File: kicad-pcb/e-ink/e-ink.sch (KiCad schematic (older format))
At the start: 0 parts

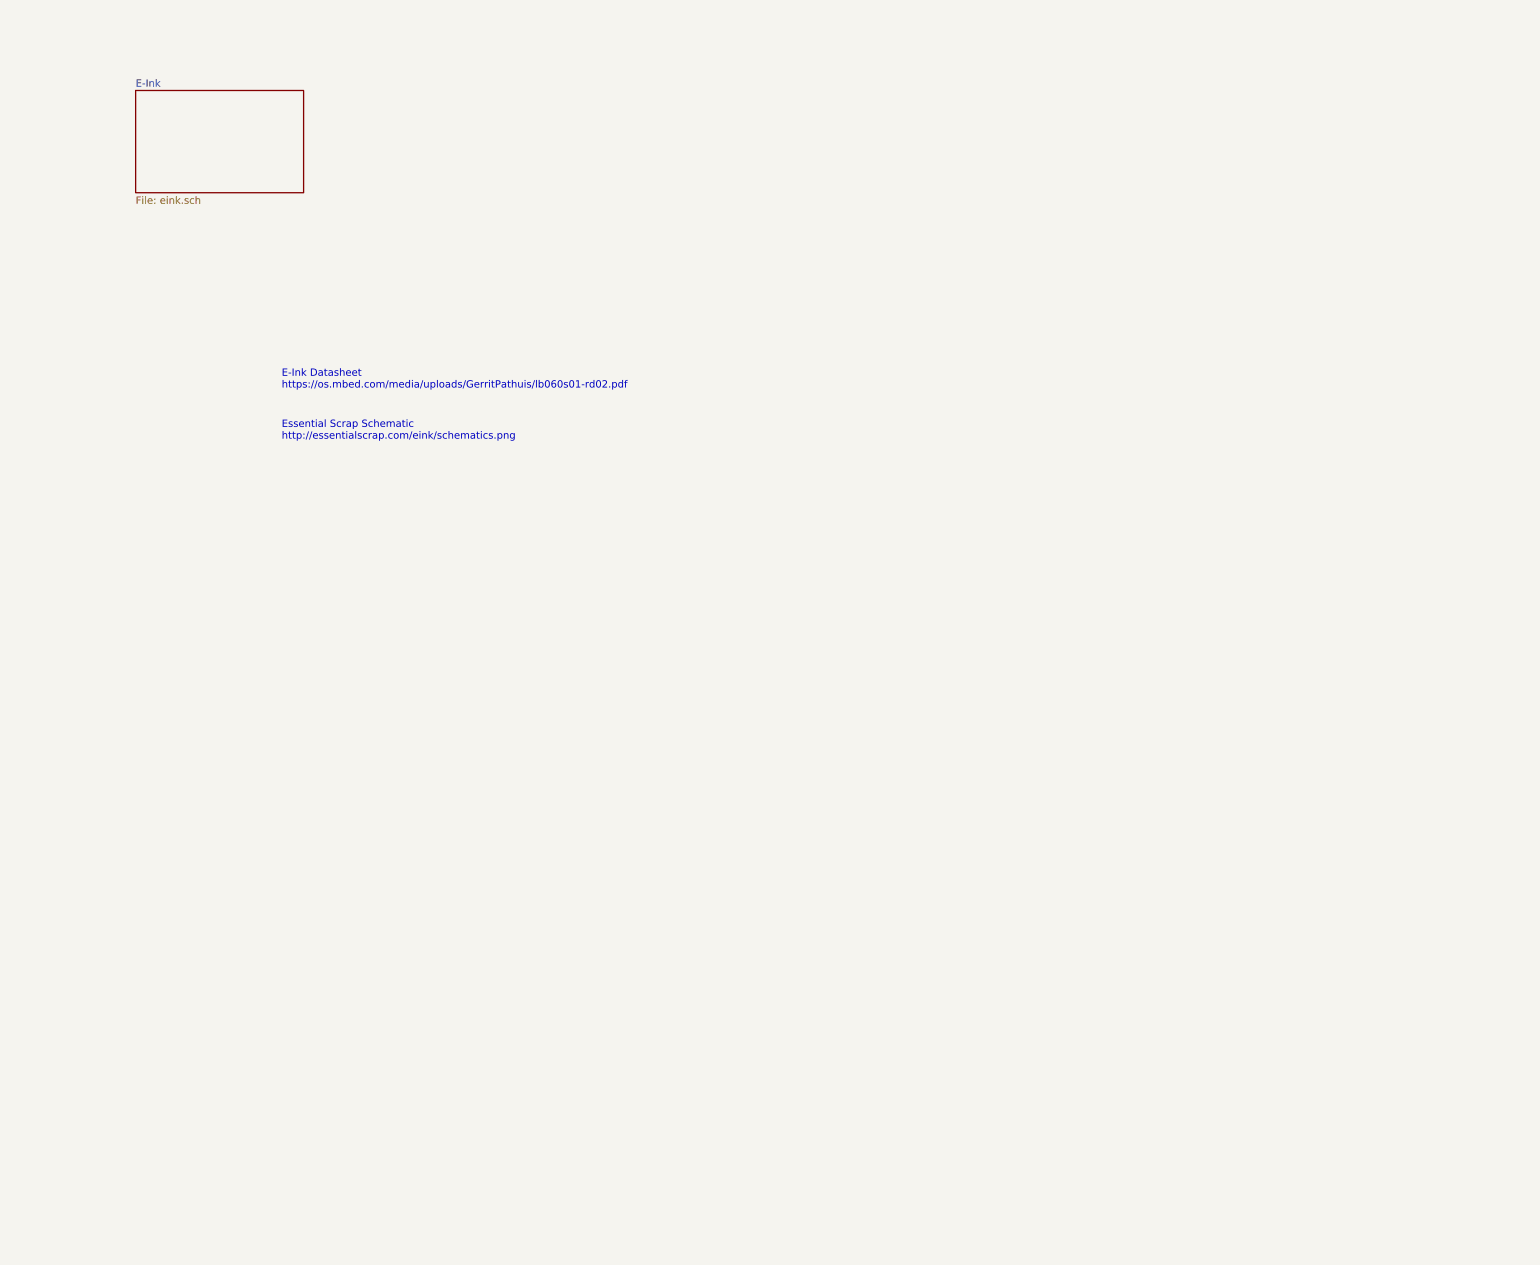
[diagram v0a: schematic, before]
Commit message: recovered from an unplanned poweroff, and removed backup files
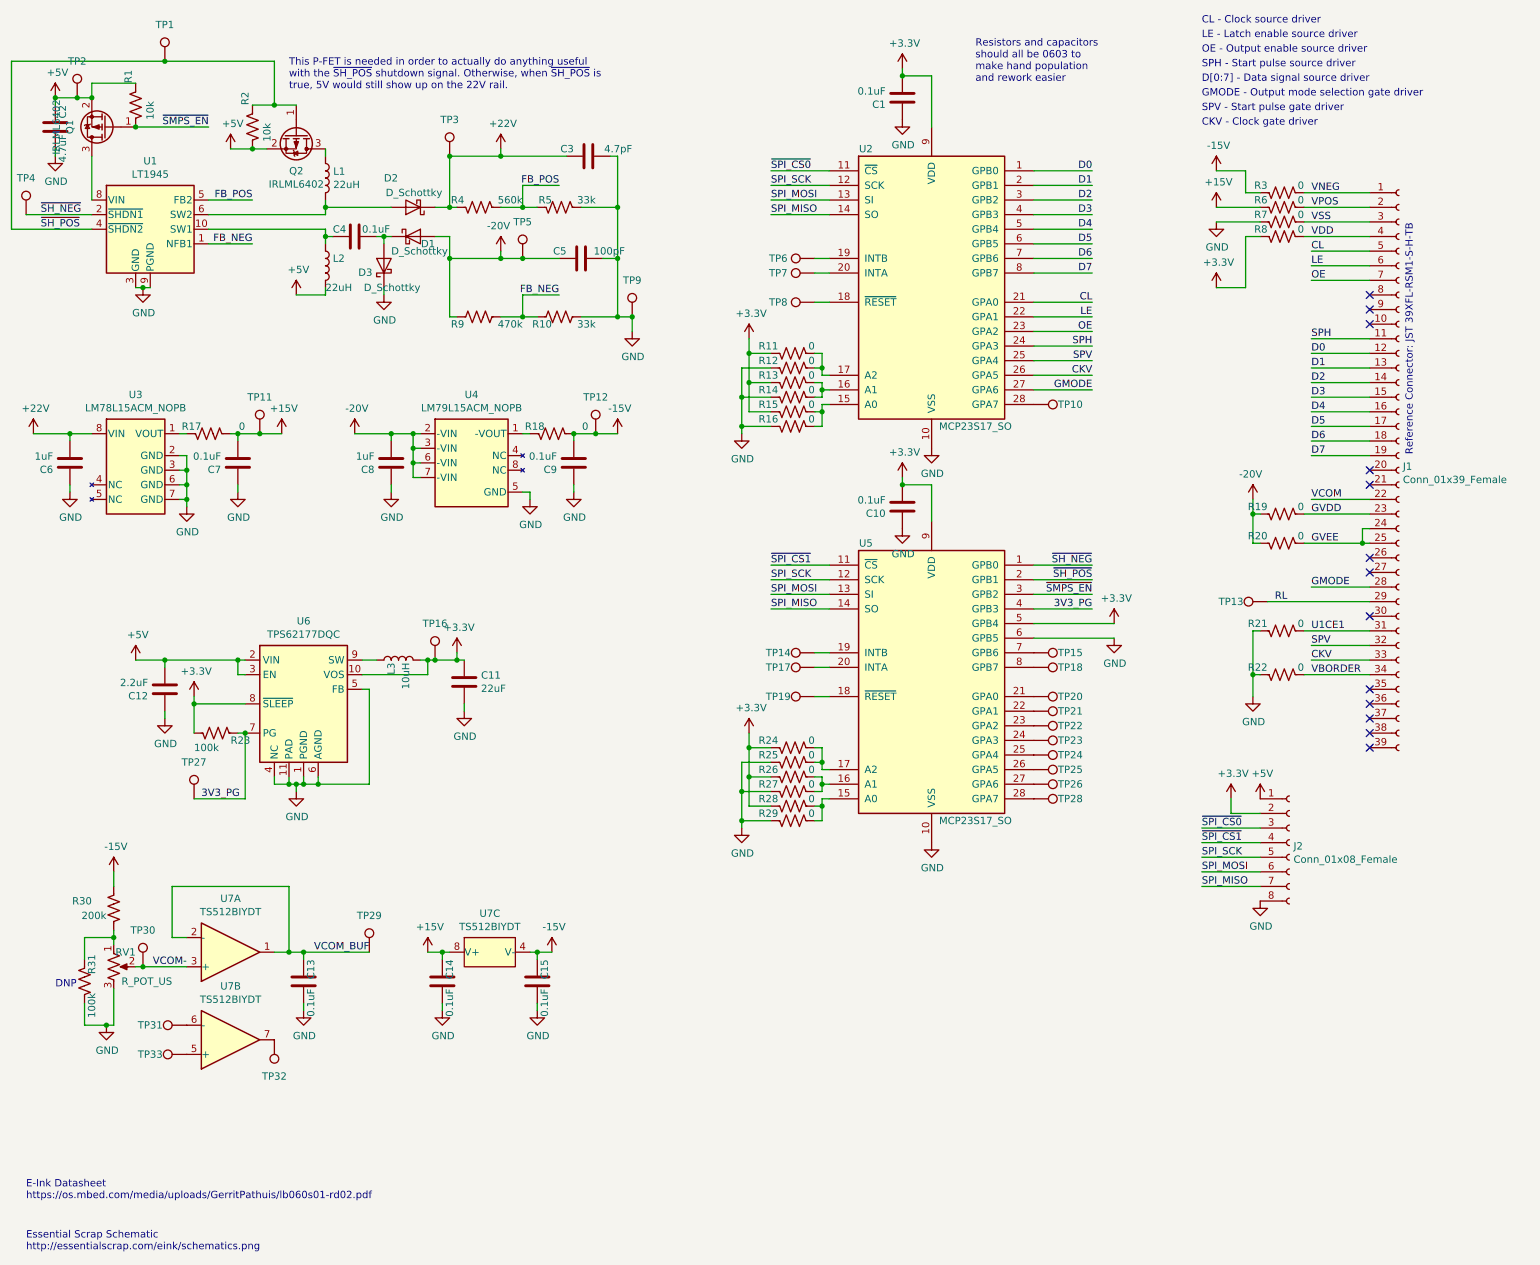
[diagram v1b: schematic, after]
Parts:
- added C1, C10, C13, C14, C15, C4, C7, C9: 0.1uF, Capacitor_SMD:C_0402_1005Metric, symbol Device:C
- added C11: 22uF, Capacitor_SMD:C_0402_1005Metric, symbol Device:C
- added C12: 2.2uF, Capacitor_SMD:C_0402_1005Metric, symbol Device:C
- added C2: 4.7uF, Capacitor_SMD:C_0402_1005Metric, symbol Device:C
- added C3: 4.7pF, Capacitor_SMD:C_0402_1005Metric, symbol Device:C
- added C5: 100pF, Capacitor_SMD:C_0402_1005Metric, symbol Device:C
- added C6, C8: 1uF, Capacitor_SMD:C_0402_1005Metric, symbol Device:C
- added D1, D2, D3: D_Schottky, symbol Device:D_Schottky
- added J1: Conn_01x39_Female, symbol Connector:Conn_01x39_Female
- added J2: Conn_01x08_Female, symbol Connector:Conn_01x08_Female
- added L1, L2: 22uH, symbol Device:L
- added L3: 10uH, symbol Device:L
- added Q1, Q2: IRLML6402, Package_TO_SOT_SMD:SOT-23, symbol Transistor_FET:IRLML6402
- added R1, R2: 10k, Resistor_SMD:R_0402_1005Metric, symbol Device:R_US
- added R10, R5: 33k, Resistor_SMD:R_0402_1005Metric, symbol Device:R_US
- added R11, R12, R13, R14, R15, R16, R17, R18, R19, R20, R21, R22, R24, R25, R26, R27, R28, R29, R3, R6, R7, R8: 0, Resistor_SMD:R_0402_1005Metric, symbol Device:R_US
- added R23, R31: 100k, Resistor_SMD:R_0402_1005Metric, symbol Device:R_US
- added R30: 200k, Resistor_SMD:R_0402_1005Metric, symbol Device:R_US
- added R4: 560k, Resistor_SMD:R_0402_1005Metric, symbol Device:R_US
- added R9: 470k, Resistor_SMD:R_0402_1005Metric, symbol Device:R_US
- added RV1: R_POT_US, symbol Device:R_POT_US
- added TP1, TP10, TP11, TP12, TP13, TP14, TP15, TP16, TP17, TP18, TP19, TP2, TP20, TP21, TP22, TP23, TP24, TP25, TP26, TP27, TP28, TP29, TP3, TP30, TP31, TP32, TP33, TP4, TP5, TP6, TP7, TP8, TP9: TestPoint, symbol Connector:TestPoint
- added U1: LT1945, Package_SO:MSOP-10_3x3mm_P0.5mm, symbol Regulator_Switching:LT1945
- added U2, U5: MCP23S17_SO, Package_SO:SOIC-28W_7.5x17.9mm_P1.27mm, symbol Interface_Expansion:MCP23S17_SO
- added U3: LM78L15ACM_NOPB, symbol custom:LM78L15ACM_NOPB
- added U4: LM79L15ACM_NOPB, symbol custom:LM79L15ACM_NOPB
- added U6: TPS62177DQC, Package_SON:WSON-10-1EP_2x3mm_P0.5mm_EP0.84x2.4mm_ThermalVias, symbol Regulator_Switching:TPS62177DQC
- added U7: TS512BIYDT, symbol custom:TS512BIYDT
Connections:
- new net: C4.2, L2.1, U1.10 (SW1)
- new net: D1.2 (A), L1.2, U1.6 (SW2)
- new net: Q1.3 (D), U1.8 (VIN)
- new net: C4.1, D2.1 (K), D3.2 (A)
- new net: L1.1, Q2.3 (D)
- new net: TP33.1, U7.5 (+)
- new net: TP31.1, U7.6 (-)
- new net: TP32.1, U7.7
- new net: R30.2, R31.1, RV1.1
- new net: R17.1, U3.1 (VOUT)
- new net: R18.1, U4.1 (-VOUT)
- new net: L3.1, U6.9 (SW)
- new net: R15.2, R16.2, U2.15 (A0)
- new net: R13.2, R14.2, U2.16 (A1)
- new net: R11.2, R12.2, U2.17 (A2)
- new net: TP8.1, U2.18 (~RESET~)
- new net: TP6.1, U2.19 (INTB)
- new net: TP7.1, U2.20 (INTA)
- new net: TP10.1, U2.28 (GPA7)
- new net: R28.2, R29.2, U5.15 (A0)
- new net: R26.2, R27.2, U5.16 (A1)
- new net: R24.2, R25.2, U5.17 (A2)
- new net: TP19.1, U5.18 (~RESET~)
- new net: TP14.1, U5.19 (INTB)
- new net: TP17.1, U5.20 (INTA)
- new net: TP20.1, U5.21 (GPA0)
- new net: TP21.1, U5.22 (GPA1)
- new net: TP22.1, U5.23 (GPA2)
- new net: TP23.1, U5.24 (GPA3)
- new net: TP24.1, U5.25 (GPA4)
- new net: TP25.1, U5.26 (GPA5)
- new net: TP26.1, U5.27 (GPA6)
- new net: TP28.1, U5.28 (GPA7)
- new net: TP15.1, U5.7 (GPB6)
- new net: TP18.1, U5.8 (GPB7)
- new net +15V: C14.2, C7.2, R17.2, R6.1, TP11.1, U7.8 (V+)
- new net +22V: C3.1, C6.2, D1.1 (K), R4.1, TP3.1, U3.8 (VIN)
- new net +3V3: C1.2, C10.2, C11.1, J2.2 (Pin_2), L3.2, R11.1, R13.1, R15.1, R23.2, R24.1, R26.1, R28.1, R8.1, TP16.1, U2.9 (VDD), U5.5 (GPB4), U5.9 (VDD), U6.10 (VOS), U6.8 (~SLEEP)
- new net +5V: C12.2, C2.2, J2.1 (Pin_1), L2.2, Q1.2 (S), Q2.2 (S), R1.1, R2.2, TP2.1, U6.2 (VIN), U6.3 (EN)
- new net -15V: C15.2, C9.2, R18.2, R3.1, R30.1, TP12.1, U7.4 (V-)
- new net -20V: C5.1, C8.2, D2.2 (A), R19.1, R20.1, R9.1, TP5.1, U4.2 (-VIN), U4.3 (-VIN), U4.6 (-VIN), U4.7 (-VIN)
- new net 3V3_PG: R23.1, TP27.1, U5.4 (GPB3), U6.7 (PG)
- new net CKV: J1.33 (Pin_33), U2.26 (GPA5)
- new net CL: J1.5 (Pin_5), U2.21 (GPA0)
- new net D0: J1.12 (Pin_12), U2.1 (GPB0)
- new net D1: J1.13 (Pin_13), U2.2 (GPB1)
- new net D2: J1.14 (Pin_14), U2.3 (GPB2)
- new net D3: J1.15 (Pin_15), U2.4 (GPB3)
- new net D4: J1.16 (Pin_16), U2.5 (GPB4)
- new net D5: J1.17 (Pin_17), U2.6 (GPB5)
- new net D6: J1.18 (Pin_18), U2.7 (GPB6)
- new net D7: J1.19 (Pin_19), U2.8 (GPB7)
- new net FB_NEG: R10.1, R9.2, U1.1 (NFB1)
- new net FB_POS: R4.2, R5.1, U1.5 (FB2)
- new net GMODE: J1.28 (Pin_28), U2.27 (GPA6)
- new net GND: C1.1, C10.1, C11.2, C12.1, C13.1, C14.1, C15.1, C2.1, C3.2, C5.2, C6.1, C7.1, C8.1, C9.1, D3.1 (K), J2.8 (Pin_8), R10.2, R12.1, R14.1, R16.1, R21.1, R22.1, R25.1, R27.1, R29.1, R31.2, R5.2, R7.1, RV1.3, TP9.1, U1.3 (GND), U1.7 (PGND), U1.9 (PGND), U2.10 (VSS), U3.2 (GND), U3.3 (GND), U3.6 (GND), U3.7 (GND), U4.5 (GND), U5.10 (VSS), U5.6 (GPB5), U6.1 (PGND), U6.11 (PAD), U6.4 (NC), U6.5 (FB), U6.6 (AGND)
- new net GVDD: J1.23 (Pin_23), R19.2
- new net GVEE: J1.24 (Pin_24), J1.25 (Pin_25), R20.2
- new net LE: J1.6 (Pin_6), U2.22 (GPA1)
- new net OE: J1.7 (Pin_7), U2.23 (GPA2)
- new net RL: J1.29 (Pin_29), TP13.1
- new net SPH: J1.11 (Pin_11), U2.24 (GPA3)
- new net SPI_MISO: J2.7 (Pin_7), U2.14 (SO), U5.14 (SO)
- new net SPI_MOSI: J2.6 (Pin_6), U2.13 (SI), U5.13 (SI)
- new net SPI_SCK: J2.5 (Pin_5), U2.12 (SCK), U5.12 (SCK)
- new net SPV: J1.32 (Pin_32), U2.25 (GPA4)
- new net U1CE1: J1.31 (Pin_31), R21.2
- new net VBORDER: J1.34 (Pin_34), R22.2
- new net VCOM: J1.22 (Pin_22)
- new net VCOM-: RV1.2, TP30.1, U7.3 (+)
- new net VCOM_BUF: C13.2, TP29.1, U7.1, U7.2 (-)
- new net VDD: J1.4 (Pin_4), R8.2
- new net VNEG: J1.1 (Pin_1), R3.2
- new net VPOS: J1.2 (Pin_2), R6.2
- new net VSS: J1.3 (Pin_3), R7.2
- new net ~SH_NEG: TP4.1, U1.2 (~SHDN1), U5.1 (GPB0)
- new net ~SH_POS: Q2.1 (G), R2.1, TP1.1, U1.4 (~SHDN2), U5.2 (GPB1)
- new net ~SMPS_EN: Q1.1 (G), R1.2, U5.3 (GPB2)
- new net ~SPI_CS0: J2.3 (Pin_3), U2.11 (~CS~)
- new net ~SPI_CS1: J2.4 (Pin_4), U5.11 (~CS~)
- no-connect marks 0 -> 13
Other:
- note added: "CKV - Clock gate driver"
- note added: "CL - Clock source driver"
- note added: "DNP"
- note added: "D[0:7] - Data signal source driver"
- note added: "GMODE - Output mode selection gate driver"
- note added: "LE - Latch enable source driver"
- note added: "OE - Output enable source driver"
- note added: "Reference Connector: JST 39XFL-RSM1-S-H-TB"
- note added: "Resistors and capacitors\nshould all be 0603 to\nmake hand population\nand rework easier"
- note added: "SPH - Start pulse source driver"
- note added: "SPV - Start pulse gate driver"
- note added: "This P-FET is needed in order to actually do anything useful \nwith the ~SH_POS~ shutdown signal. Otherwise, when ~SH_POS~ is \ntrue, 5V would still show up on the 22V rail."
